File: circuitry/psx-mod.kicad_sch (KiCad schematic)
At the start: 52 parts, among them J1 Conn_01x04, J10 USB 2.0 Type-C, J11 Conn_01x04, J12 Conn_01x01, J13 Conn_01x01, J4 Conn_01x02, J5 Conn_01x02, J6 Conn_01x01, J7 Conn_01x01, J8 Conn_01x02, J9 Conn_01x04, U1 ATtiny404-SS, U2 Si5351A-B-GT, U3 USBLC6-2SC6, U4 CH340C, U5 74LVC2G04, U6 74LVC2G04, U7 XC6219B332MR, Y1 27MHz

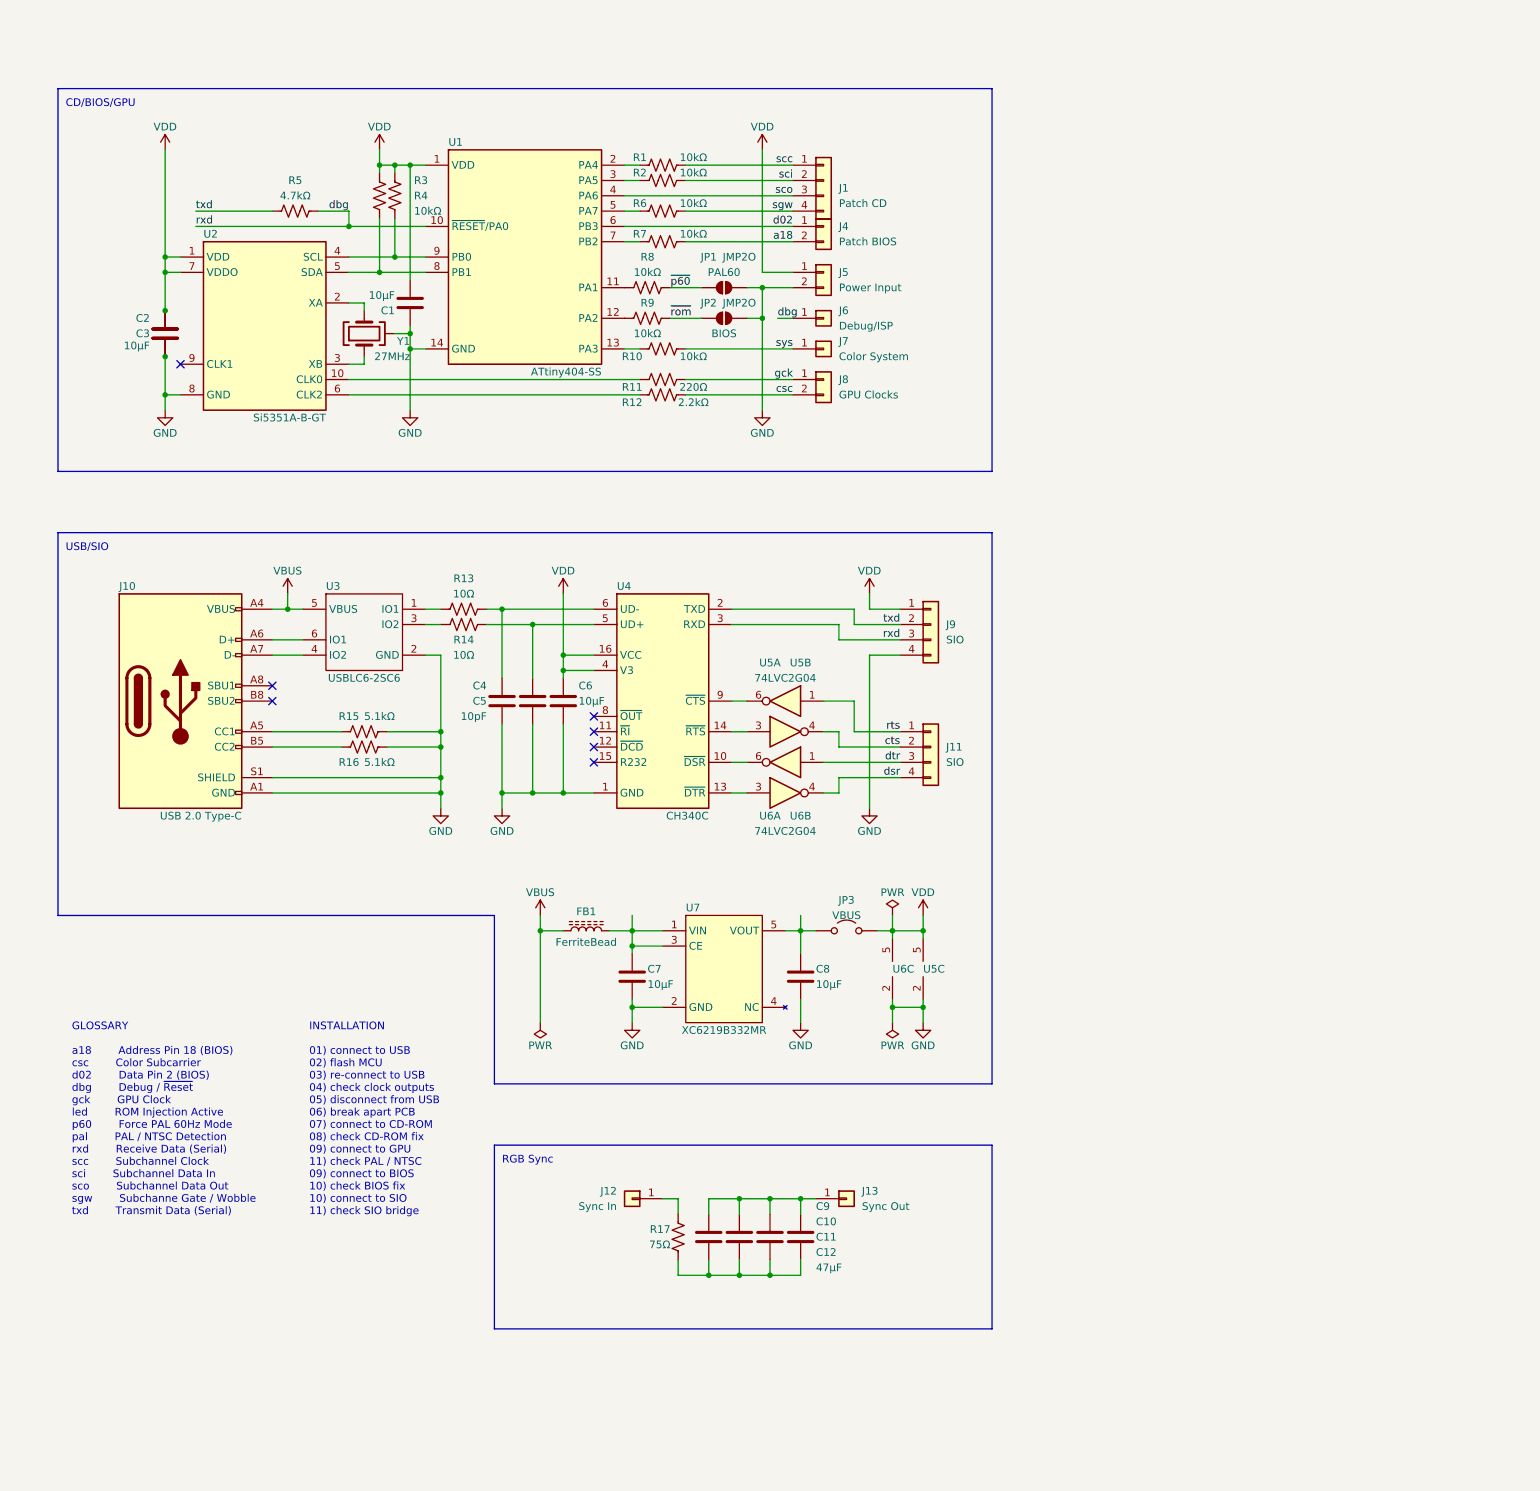
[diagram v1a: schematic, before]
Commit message: Completed schematic and layout.
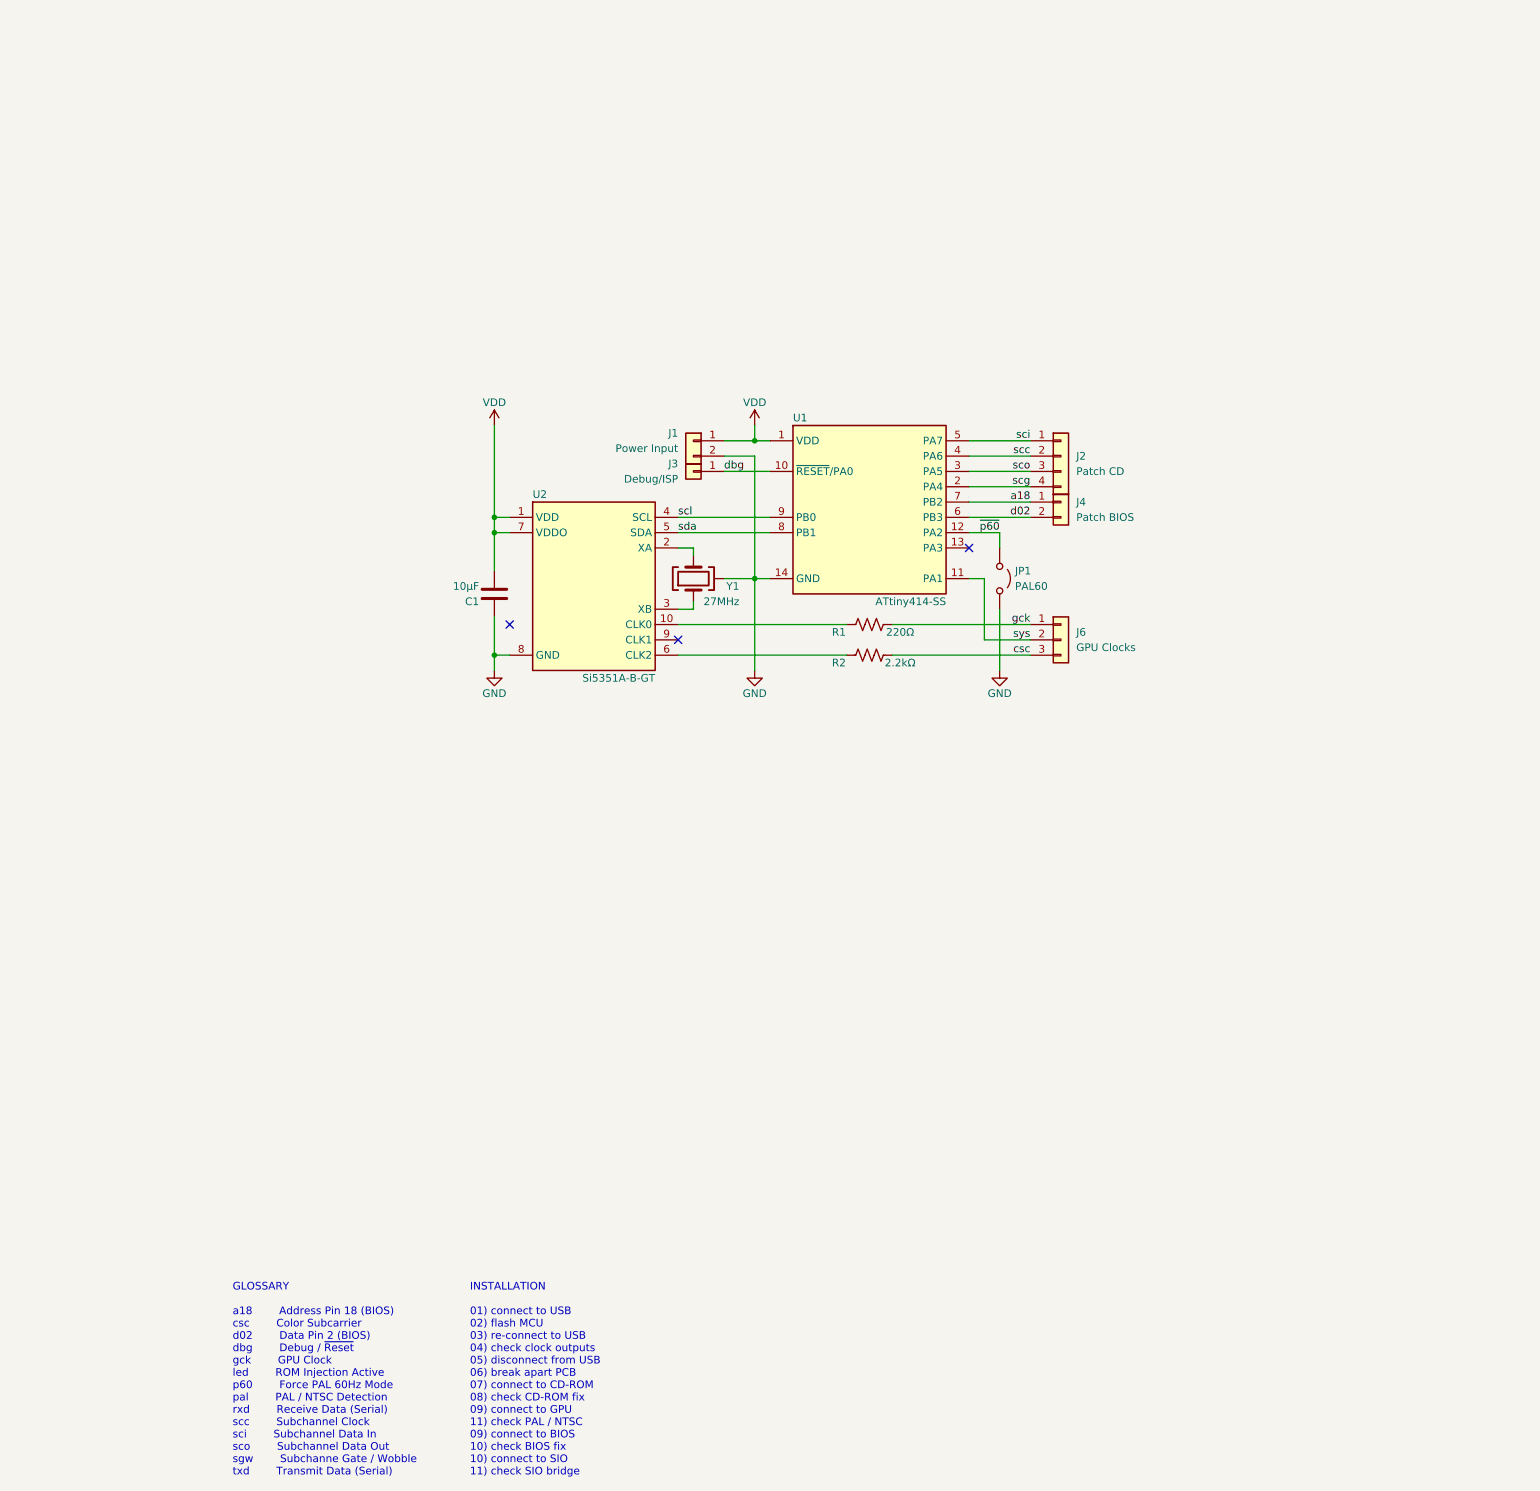
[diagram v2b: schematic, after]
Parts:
- removed C10, C11, C12, C9: 47µF, Capacitor_SMD:C_1206_3216Metric_Pad1.33x1.80mm_HandSolder, symbol Device:C
- removed C2, C3, C6, C7, C8: 10µF, Capacitor_SMD:C_0603_1608Metric_Pad1.08x0.95mm_HandSolder, symbol Device:C
- removed C4, C5: 10pF, Capacitor_SMD:C_0603_1608Metric_Pad1.08x0.95mm_HandSolder, symbol Device:C
- removed FB1: FerriteBead, Inductor_SMD:L_1206_3216Metric_Pad1.42x1.75mm_HandSolder, symbol Device:L_Ferrite
- removed J10: USB 2.0 Type-C, PSX_Mod:CONN-SMD_HX-TYPE-C-16PIN, symbol PSX_Mod:USB_C_Receptacle_USB2.0_16P
- removed J11, J9: Conn_01x04, PSX_Mod:CONN-SMD_4P, symbol Connector_Generic:Conn_01x04
- removed J12, J13, J7: Conn_01x01, PSX_Mod:CONN-SMD_1P, symbol Connector_Generic:Conn_01x01
- removed J8: Conn_01x02, PSX_Mod:CONN-SMD_2P, symbol Connector_Generic:Conn_01x02
- removed JP1, JP2: JMP2O, Jumper:SolderJumper-2_P1.3mm_Open_RoundedPad1.0x1.5mm, symbol Jumper:SolderJumper_2_Open
- removed JP3: Jumper_2_Open, Jumper:SolderJumper-2_P1.3mm_Open_RoundedPad1.0x1.5mm, symbol Jumper:Jumper_2_Open
- removed R1, R10, R2, R3, R4, R6, R7, R8, R9: 10kΩ, Resistor_SMD:R_0603_1608Metric_Pad0.98x0.95mm_HandSolder, symbol Device:R_US
- removed R13, R14: 10Ω, Resistor_SMD:R_0603_1608Metric_Pad0.98x0.95mm_HandSolder, symbol Device:R_US
- removed R15, R16: 5.1kΩ, Resistor_SMD:R_0603_1608Metric_Pad0.98x0.95mm_HandSolder, symbol Device:R_US
- removed R17: 75Ω, Resistor_SMD:R_1206_3216Metric_Pad1.30x1.75mm_HandSolder, symbol Device:R_US
- removed R5: 4.7kΩ, Resistor_SMD:R_0603_1608Metric_Pad0.98x0.95mm_HandSolder, symbol Device:R_US
- removed U3: USBLC6-2SC6, Package_TO_SOT_SMD:SOT-23-6, symbol PSX_Mod:USBLC6_2SC6
- removed U4: CH340C, Package_SO:SOIC-16_3.9x9.9mm_P1.27mm, symbol PSX_Mod:CH340C
- removed U5, U6: 74LVC2G04, Package_TO_SOT_SMD:SOT-23-6, symbol PSX_Mod:74LVC2G04
- removed U7: XC6219B332MR, Package_TO_SOT_SMD:SOT-23-5, symbol PSX_Mod:XC6219B332MR
- added J6: Conn_01x03, PSX_Mod:CONN-SMD_3P, symbol Connector_Generic:Conn_01x03
- added JP1: Jumper_2_Open, Jumper:SolderJumper-2_P1.3mm_Open_RoundedPad1.0x1.5mm, symbol Jumper:Jumper_2_Open
- U1: value ATtiny404-SS -> ATtiny414-SS; symbol PSX_Mod:ATtiny404-SS -> PSX_Mod:ATtiny414-SS
- renumbered J5 to J1, J1 to J2, J6 to J3, R11 to R1, R12 to R2
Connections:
- net sgw is gone; now on net scg: J2.4 (Pin_4)
- net GND: now also JP1.2 (B)
- net a18: now also J4.1 (Pin_1), U1.7 (PB2); no longer J4.2 (Pin_2)
- net csc: now also J6.3 (Pin_3)
- net d02: now also J4.2 (Pin_2); no longer J4.1 (Pin_1)
- net gck: now also J6.1 (Pin_1)
- net scc: now also J2.2 (Pin_2), U1.4 (PA6); no longer J2.1 (Pin_1)
- net sci: now also J2.1 (Pin_1), U1.5 (PA7); no longer J2.2 (Pin_2)
- net sco: now also U1.3 (PA5); no longer U1.4 (PA6)
- net sys: now also U1.11 (PA1), J6.2 (Pin_2)
- net ~{p60}: now also U1.12 (PA2), JP1.1 (A)
- net scg: now reaches U1.2 (PA4)
- net sda: now reaches U1.8 (PB1), U2.5 (SDA)
- net scl: now reaches U1.9 (PB0), U2.4 (SCL)
- no-connect marks 7 -> 3
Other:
- note removed: "CD/BIOS/GPU"
- note removed: "RGB Sync"
- note removed: "USB/SIO"
- moved on the sheet: C1, J1, J2, J3, J4, R1, R2, U1, U2, Y1
